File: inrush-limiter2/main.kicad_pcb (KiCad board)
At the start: 2 copper layers, 33 parts, among them K1 RELAY_2RT, P1 CONN_01X04, P2 CONN_01X02, Q1 2N3904, Q2 PN2222A, T1 MY-TRANSFO, U1 LM393, U2 50 ohm NTC

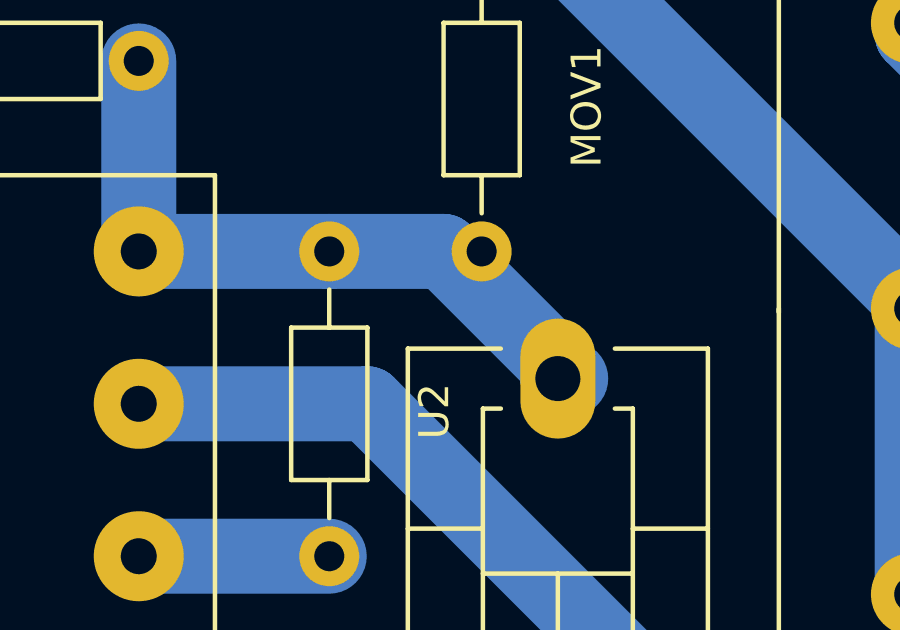
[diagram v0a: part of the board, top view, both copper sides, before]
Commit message: yes its needed
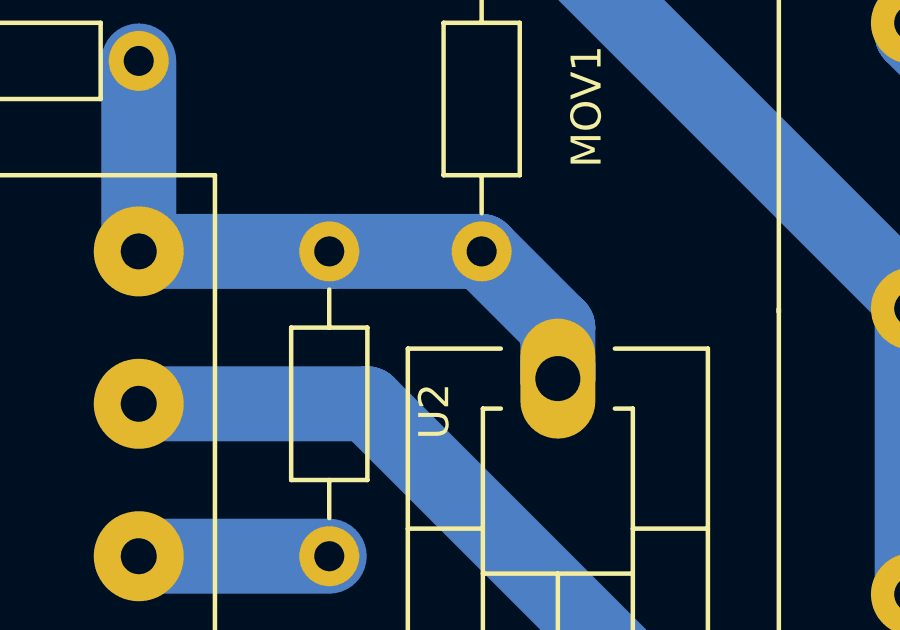
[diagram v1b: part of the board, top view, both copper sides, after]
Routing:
- net AC-live-f: track 23.2 -> 23.9 mm
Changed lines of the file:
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@@
   (general
     (links 59)
-    (no_connects 1)
-    (area -3.275001 -6.42512 234.358001 96.28099)
+    (no_connects 0)
+    (area 110.105 47.685 234.358001 96.28099)
     (thickness 1.6)
     (drawings 0)
@@
   (segment (start 123.19254 67.31052) (end 123.19 67.30798) (width 1) (layer B.Cu) (net 2) (status 30))
   (segment (start 146.04798 69.85) (end 146.04746 69.84948) (width 1) (layer B.Cu) (net 2) (status 30))
+  (segment (start 207.01 70.27926) (end 207.01 68.58) (width 2.5) (layer B.Cu) (net 3) (status C00000))
+  (segment (start 207.01 68.58) (end 204.47 66.04) (width 2.5) (layer B.Cu) (net 3) (status C00000))
+  (segment (start 204.47 66.04) (end 199.39 66.04) (width 2.5) (layer B.Cu) (net 3) (status C00000))
   (segment (start 193.04 66.04) (end 193.04 59.69) (width 2.5) (layer B.Cu) (net 3) (status 30))
   (segment (start 207.01 70.27926) (end 207.01 69.85) (width 2.5) (layer B.Cu) (net 3) (status 30))
-  (segment (start 207.01 69.85) (end 203.2 66.04) (width 2.5) (layer B.Cu) (net 3) (status 10))
-  (segment (start 203.2 66.04) (end 199.39 66.04) (width 2.5) (layer B.Cu) (net 3) (status 20))
   (segment (start 207.01 70.27926) (end 207.01 69.85) (width 2.5) (layer B.Cu) (net 3) (status 30))
   (segment (start 199.39 66.04) (end 193.04 66.04) (width 2.5) (layer B.Cu) (net 3) (status 30))
-  (segment (start 207.01 70.27926) (end 207.43926 70.27926) (width 2.5) (layer B.Cu) (net 3) (status 30))
   (segment (start 157.56128 63.5) (end 153.67 63.5) (width 1) (layer B.Cu) (net 4) (status 10))
   (segment (start 151.13 57.15) (end 152.4 58.42) (width 1) (layer B.Cu) (net 4))
